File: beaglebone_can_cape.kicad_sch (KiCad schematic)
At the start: 8 parts, among them J1 DCAN0, J2 DCAN1, P8 BeagleBone_Black_Header, P9 BeagleBone_Black_Header, U1 TCAN332, U2 TCAN332

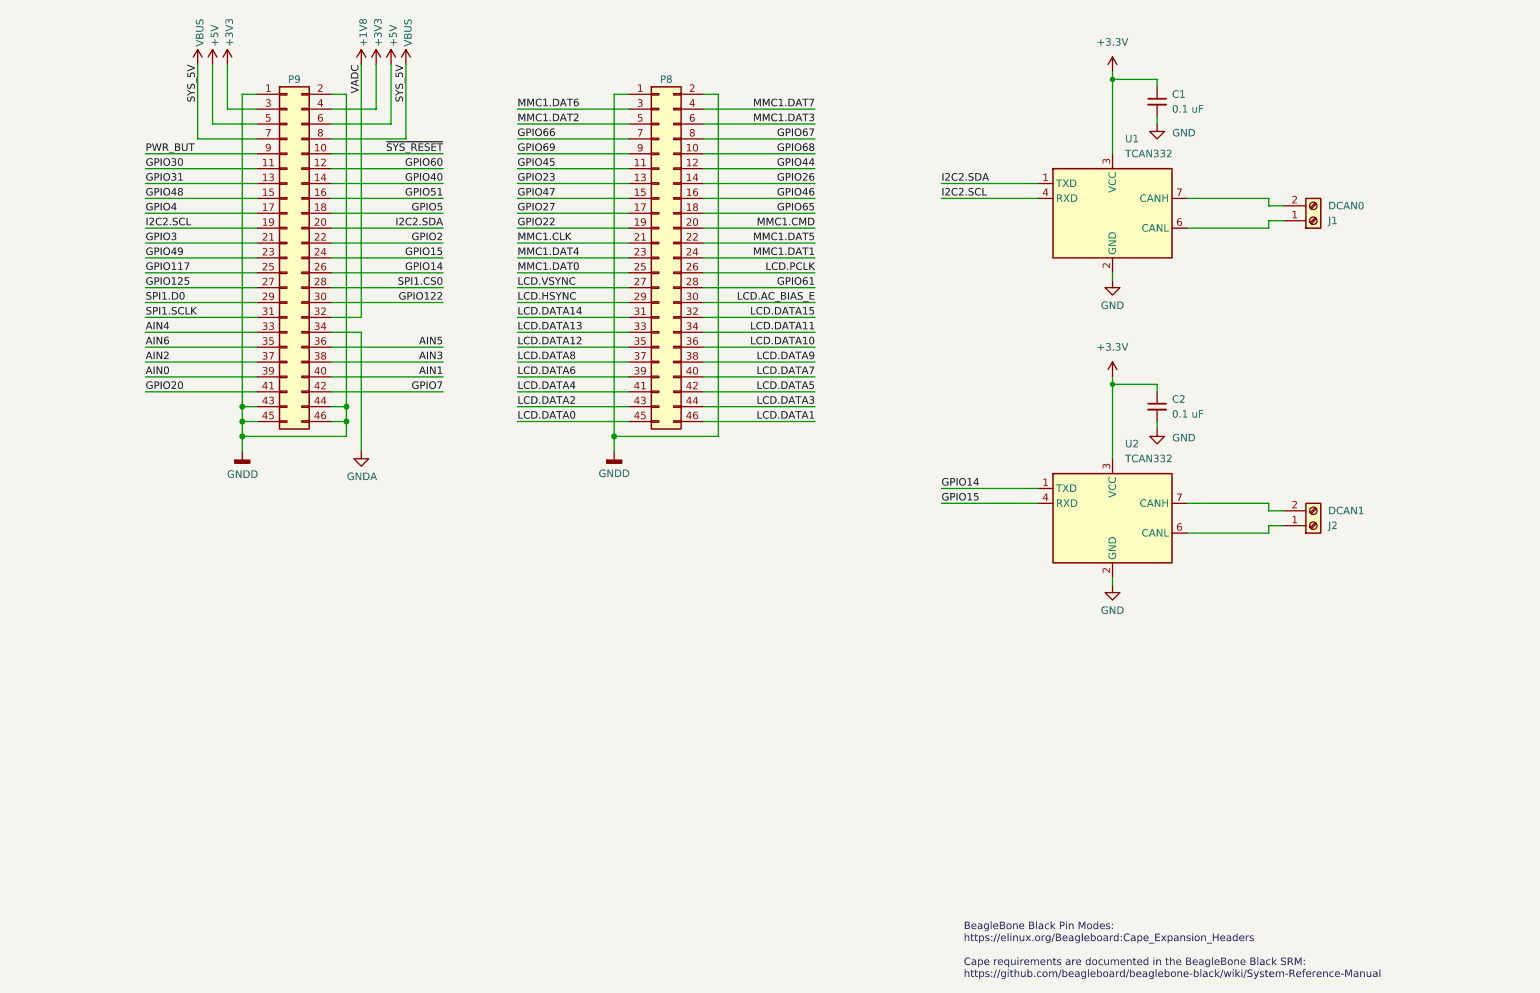
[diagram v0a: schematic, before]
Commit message: finished sch, adding footprints now
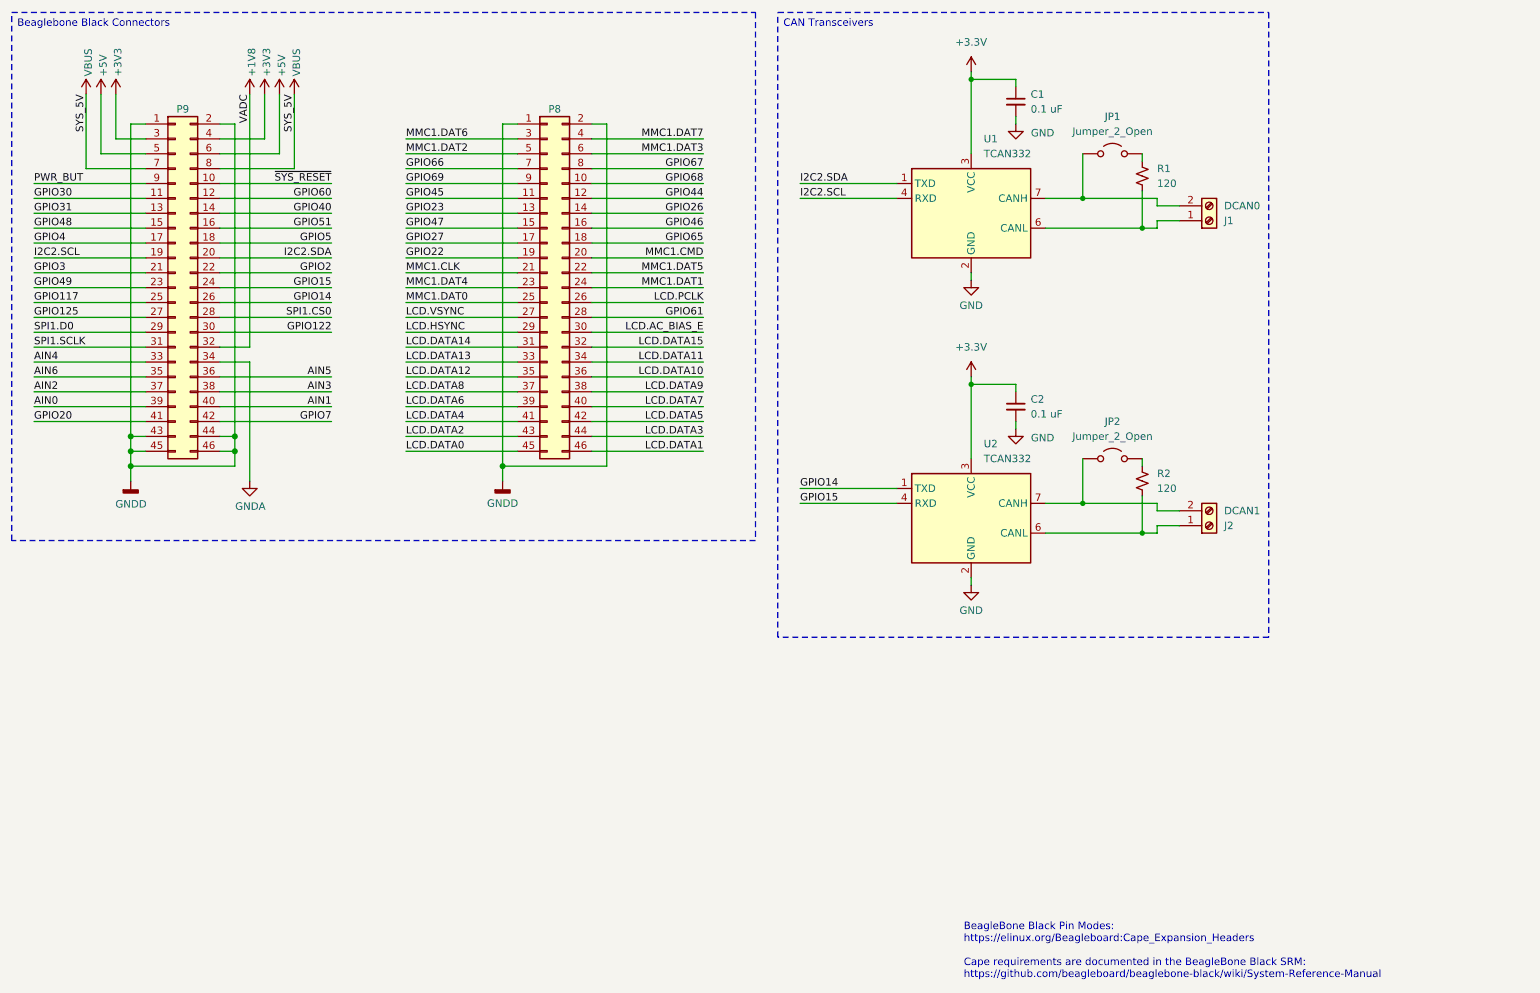
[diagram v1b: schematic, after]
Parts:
- added JP1, JP2: Jumper_2_Open, Connector_PinHeader_2.54mm:PinHeader_1x02_P2.54mm_Vertical, symbol Jumper:Jumper_2_Open
- added R1, R2: 120, symbol Device:R_Small_US
- J1, J2: footprint (none) -> TerminalBlock_RND:TerminalBlock_RND_205-00232_1x02_P5.08mm_Horizontal
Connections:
- net at J1.1 (Pin_1), U1.6 (CANL): now also R1.2
- net at J1.2 (Pin_2), U1.7 (CANH): now also JP1.1 (A)
- net at J2.1 (Pin_1), U2.6 (CANL): now also R2.2
- net at J2.2 (Pin_2), U2.7 (CANH): now also JP2.1 (A)
- new net: JP1.2 (B), R1.1
- new net: JP2.2 (B), R2.1
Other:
- moved on the sheet: C1, C2, J1, J2, P8, P9, U1, U2
